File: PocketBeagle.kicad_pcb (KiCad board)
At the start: 4 copper layers, 55 x 35 mm, 50 parts, among them SW1 POWER, U1 OSD3358-512M-BSM, U2 SN74LVC1G07DCK, U3 TPD4S012DRY, X1 10118192-0001LF, X2 MICROSD, Y1 24 MHz

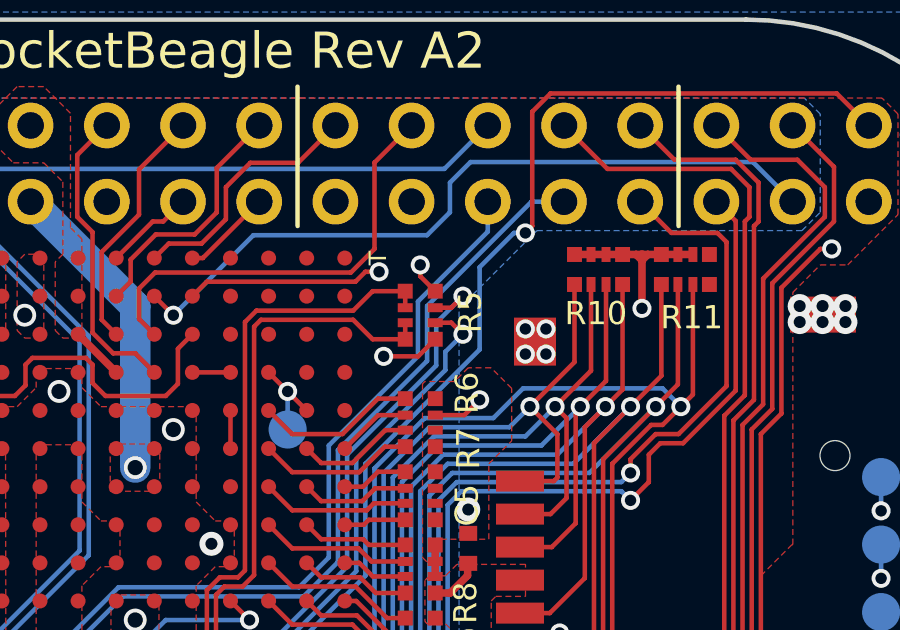
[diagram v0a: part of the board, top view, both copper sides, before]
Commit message: Update footprint references for good measure
Signed-off-by: Michael Welling <mwelling@ieee.org>
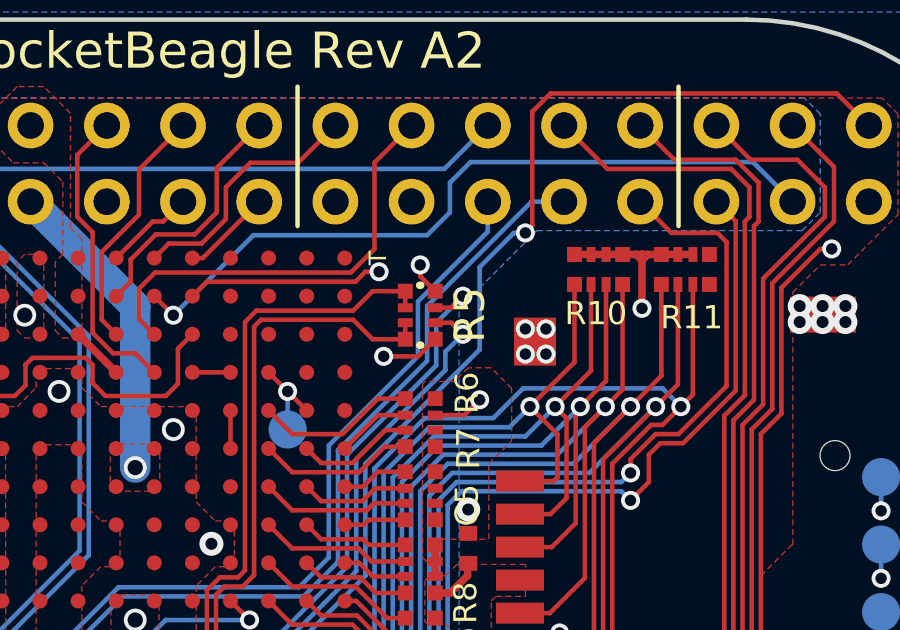
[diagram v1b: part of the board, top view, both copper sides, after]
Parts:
- C1, C2, C3, C4, C5, C7, R1, R12, R2, R3: footprint 0402 -> PocketBeagle.pretty:0402
- C6, FB1, FB2: footprint 0603 -> PocketBeagle.pretty:0603
- PWR81, USR0, USR1, USR2, USR3: footprint 0603-LED -> PocketBeagle.pretty:0603-LED
- R10, R11, R5, R6, R7, R8, R9: footprint RN0804 -> PocketBeagle.pretty:RN0804
- SW1: footprint MINI_PUSHBUTTON -> PocketBeagle.pretty:MINI_PUSHBUTTON
- TP1, TP10, TP11, TP2, TP3, TP4, TP5, TP6, TP7, TP8, TP9, WP81: footprint B1_27 -> PocketBeagle.pretty:B1_27
- U1: footprint OSD335X-BGA-256 -> PocketBeagle.pretty:OSD335X-BGA-256
- U2: footprint SC70(TI-DCK) -> PocketBeagle.pretty:SC70(TI-DCK)
- U3: footprint SON-6(TI)-DRY -> PocketBeagle.pretty:SON-6(TI)-DRY
- X1: footprint 10118192-0001LF(MICRO-USB-B-AMPHENOL-FCI) -> PocketBeagle.pretty:10118192-0001LF(MICRO-USB-B-AMPHENOL-FCI)
- X2: footprint MICROSD -> PocketBeagle.pretty:MICROSD
- Y1: footprint CRYSTAL_5X3.2MM -> PocketBeagle.pretty:CRYSTAL_5X3.2MM
